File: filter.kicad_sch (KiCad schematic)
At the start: 32 parts

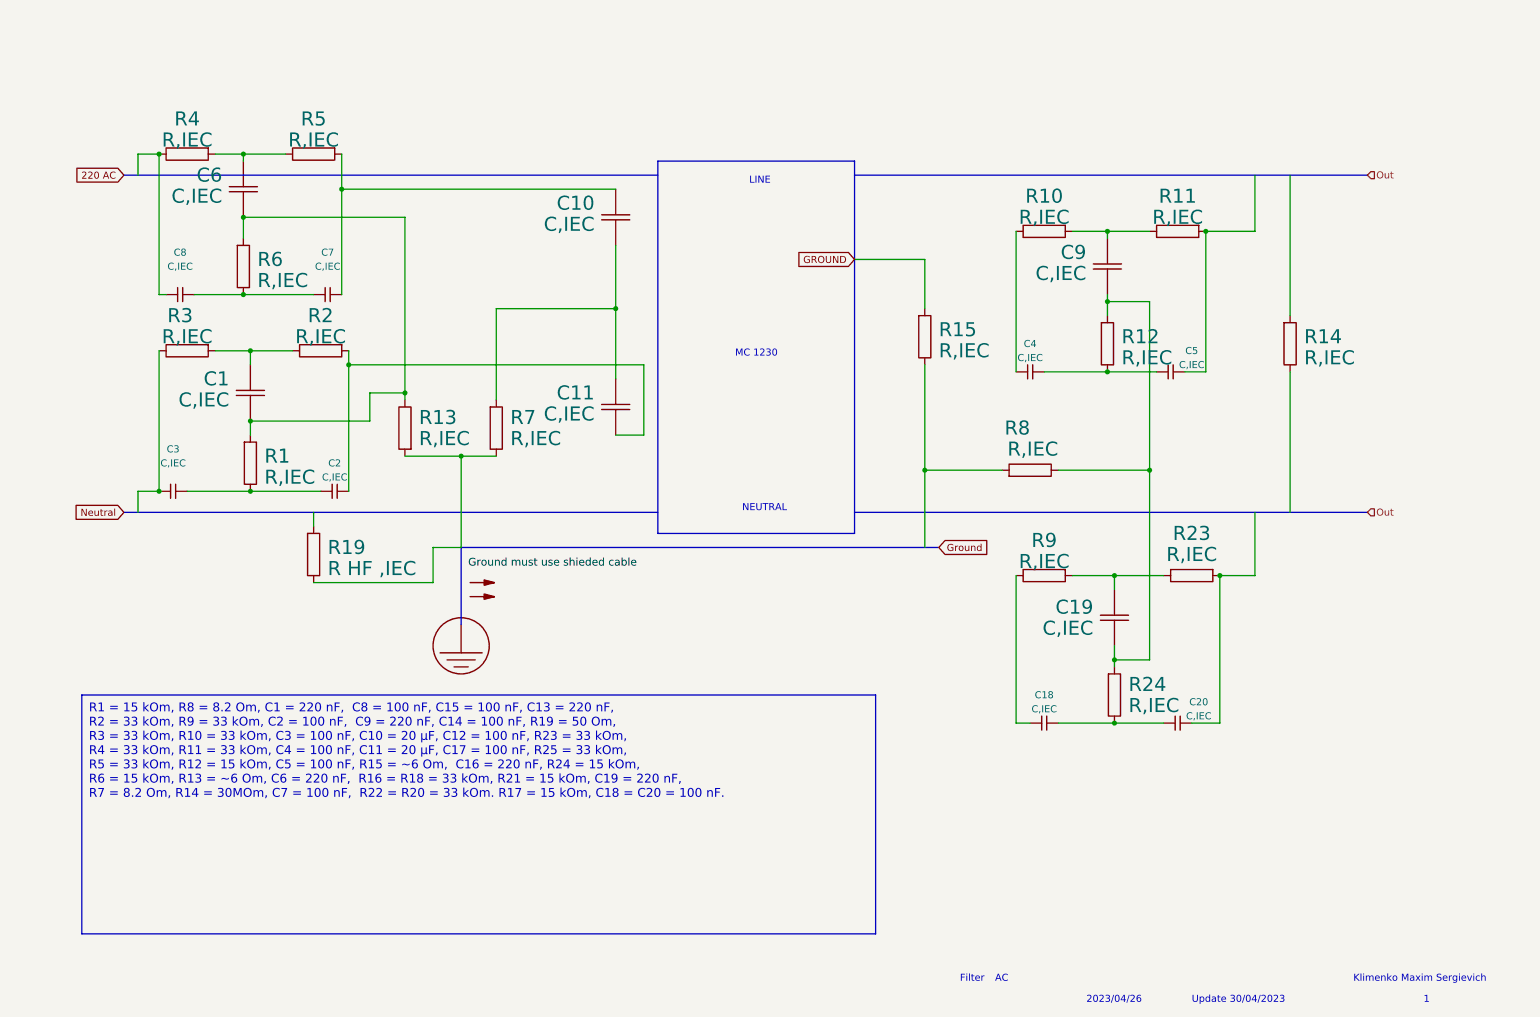
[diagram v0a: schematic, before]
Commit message: Upgrade
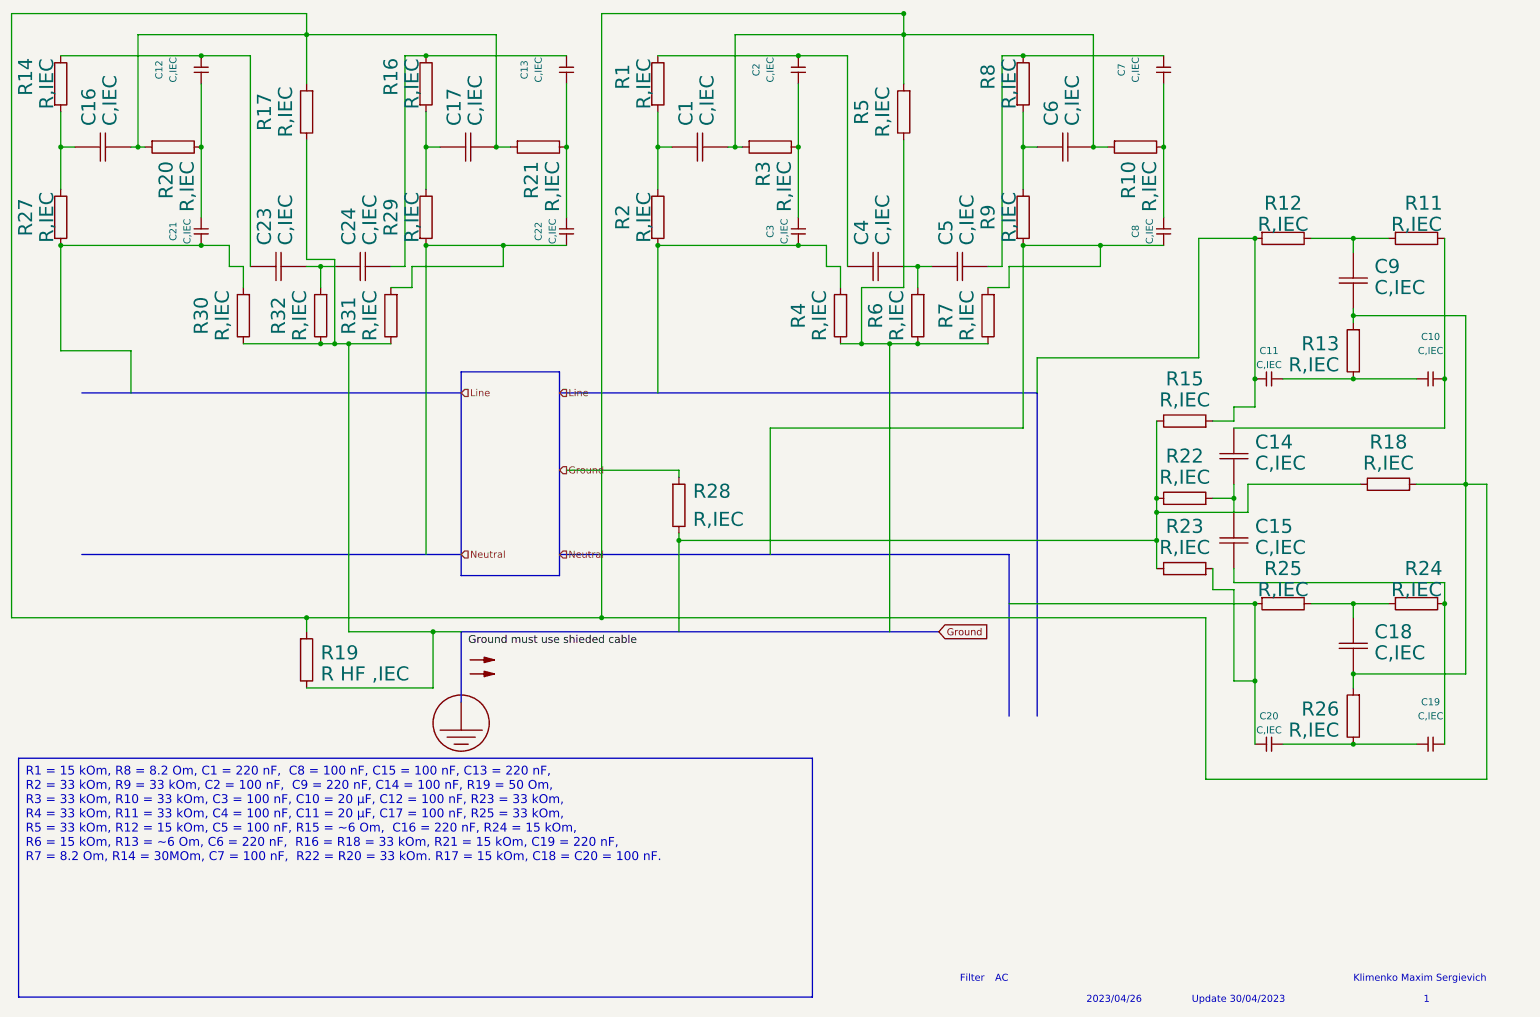
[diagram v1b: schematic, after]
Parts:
- removed C10, C11, C19: C,IEC, symbol PCM_Generic:C,IEC
- removed C18, C4, C5: C,IEC, symbol PCM_Generic-50:C,IEC
- added C10, C11, C12, C13, C19, C21, C22: C,IEC, symbol PCM_Generic-50:C,IEC
- added C14, C15, C16, C17, C18, C23, C24, C4, C5: C,IEC, symbol PCM_Generic:C,IEC
- added R16, R17, R18, R20, R21, R22, R25, R26, R27, R28, R29, R30, R31, R32: R,IEC, symbol PCM_Generic:R,IEC
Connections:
- net at C2.2 (-), R1.2 (-): now also C4.1 (+); no longer C3.1 (+)
- net at R11.1 (+): now also C9.1 (+), R12.2 (-)
- net at R5.1 (+): now also C1.2 (-), C6.2 (-), C9.2 (-), R10.1 (+), R13.1 (+), R19.1 (+), R3.1 (+), C16.2 (-), C17.2 (-), C18.2 (-), R17.1 (+), R18.1 (+), R20.1 (+), R21.1 (+), R26.1 (+); no longer C7.1 (+)
- net at R24.2 (-): now also C15.2 (-), C19.2 (-); no longer C20.2 (-)
- net at R9.2 (-): now also C6.1 (+), R8.1 (+)
- net at R7.1 (+): now also C8.1 (+), R9.1 (+)
- net at C2.1 (+): now also C3.2 (-), R3.2 (-); no longer R2.1 (+)
- net at R10.2 (-): now also C7.1 (+), C8.2 (-)
- net at R15.2 (-): now also R23.2 (-), R18.2 (-), R22.2 (-), R28.2 (-); no longer R8.1 (+)
- net at R14.1 (+): now also C16.1 (+), R27.2 (-)
- net at R14.2 (-): now also C12.2 (-), C23.1 (+)
- net at R4.2 (-): now also R5.2 (-), R6.2 (-), R7.2 (-); no longer C8.2 (-)
- net at C20.1 (+), R23.1 (+): now also R25.1 (+)
- net at C1.1 (+), R2.2 (-): now also R1.1 (+); no longer R3.1 (+)
- net GROUND: no longer names the net of R15.1 (+)
- net GROUND: now also R12.1 (+), C11.1 (+)
- new net: C18.1 (+), R24.1 (+), R25.2 (-)
- new net: C23.2 (-), C24.1 (+), R32.1 (+)
- new net: C4.2 (-), C5.1 (+), R6.1 (+)
- new net: C19.1 (+), C20.2 (-), R26.2 (-)
- new net: R17.2 (-), R19.2 (-), R30.2 (-), R31.2 (-), R32.2 (-)
- new net: C12.1 (+), C21.2 (-), R20.2 (-)
- new net: C5.2 (-), C7.2 (-), R8.2 (-)
- new net: C21.1 (+), R27.1 (+), R30.1 (+)
- new net: C10.2 (-), C14.1 (+), R11.2 (-)
- new net: C14.2 (-), C15.1 (+), R22.1 (+)
- new net: C3.1 (+), R2.1 (+), R4.1 (+)
- new net: C10.1 (+), C11.2 (-), R13.2 (-)
- new net: C13.1 (+), C22.2 (-), R21.2 (-)
- new net: C22.1 (+), R29.1 (+), R31.1 (+)
- new net: C17.1 (+), R16.1 (+), R29.2 (-)
- new net: C13.2 (-), C24.2 (-), R16.2 (-)
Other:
- note removed: "LINE"
- note removed: "MC 1230"
- note removed: "NEUTRAL"
- moved on the sheet: R19
